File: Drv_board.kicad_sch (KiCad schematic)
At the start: 31 parts, among them J1 USB_B_Micro, J3 OLED_CONN, J4 SWD, J4 WS_LED_0_CONN, J5 WS_LED_1_CONN, J6 SRF-05_CONN, J7 QTR_CONN, SW1 SW_BOOT, U2 STM32F107RCTx, U3 USBLC6-2SC6, Y3 16 MHz

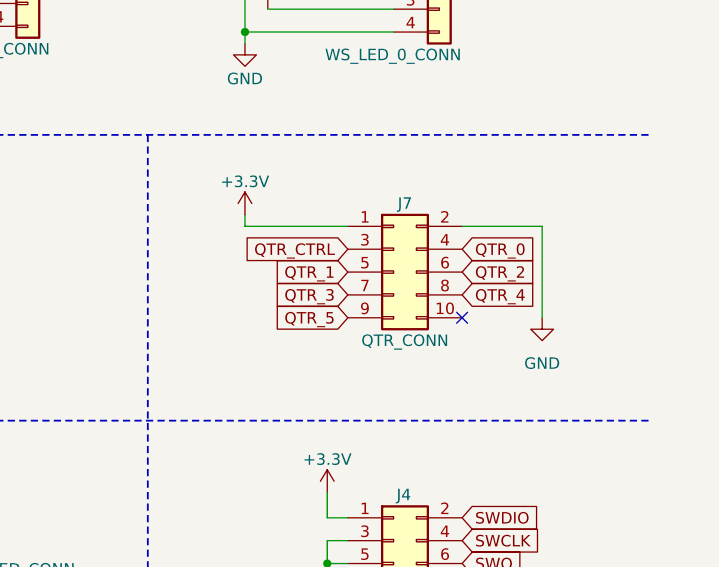
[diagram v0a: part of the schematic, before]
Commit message: more layout
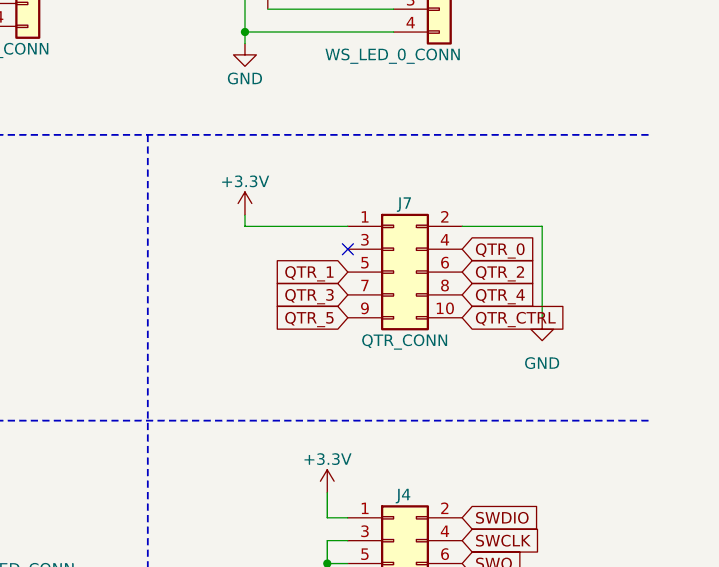
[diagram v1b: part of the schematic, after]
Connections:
- net QTR_CTRL: now also J7.10 (Pin_10); no longer J7.3 (Pin_3)
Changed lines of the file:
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@@
   (no_connect (at 115.57 85.725))
   (no_connect (at 115.57 88.265))
-  (no_connect (at 264.16 102.235))
+  (no_connect (at 251.46 94.615))
   (wire (pts (xy 249.174 124.46) (xy 251.46 124.46))
     (stroke (width 0) (type default))
@@
     )
   )
-  (global_label "QTR_CTRL" (shape input) (at 251.46 94.615 180) (fields_autoplaced)
-    (effects (font (size 1.27 1.27)) (justify right))
-    (property "Intersheetrefs" "${INTERSHEET_REFS}" (at 239.4828 94.615 0)
-      (effects (font (size 1.27 1.27)) (justify right) hide)
+  (global_label "QTR_CTRL" (shape input) (at 264.16 102.235 0) (fields_autoplaced)
+    (effects (font (size 1.27 1.27)) (justify left))
+    (property "Intersheetrefs" "${INTERSHEET_REFS}" (at 276.1372 102.235 0)
+      (effects (font (size 1.27 1.27)) (justify left) hide)
     )
   )

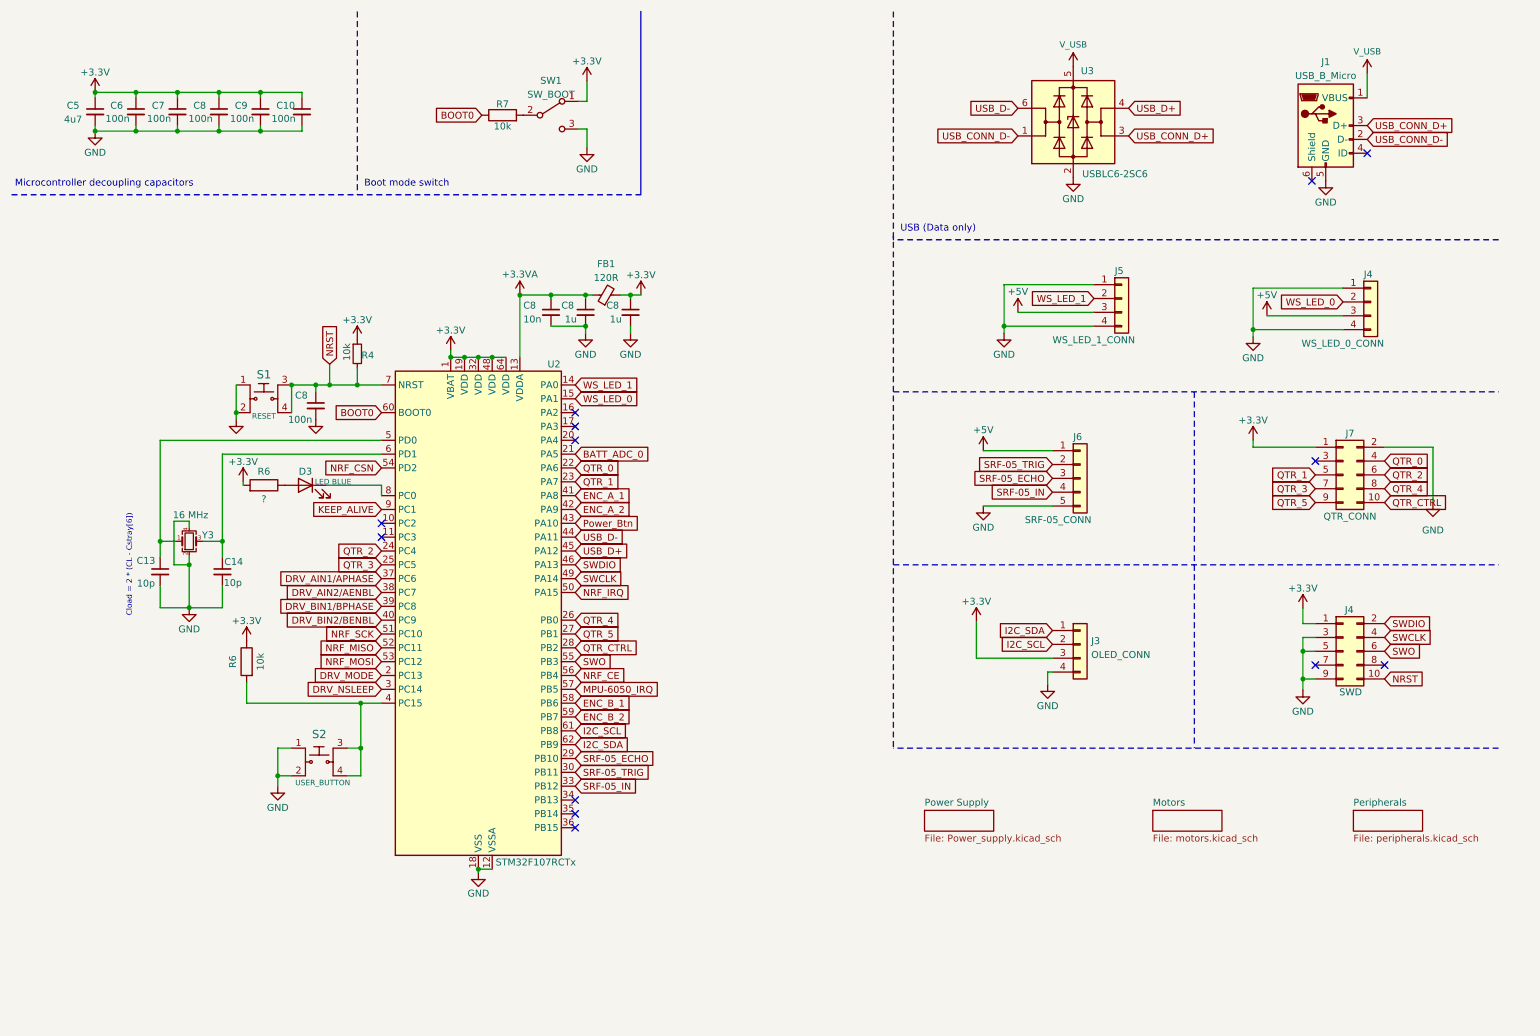
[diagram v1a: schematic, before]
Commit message: layout...
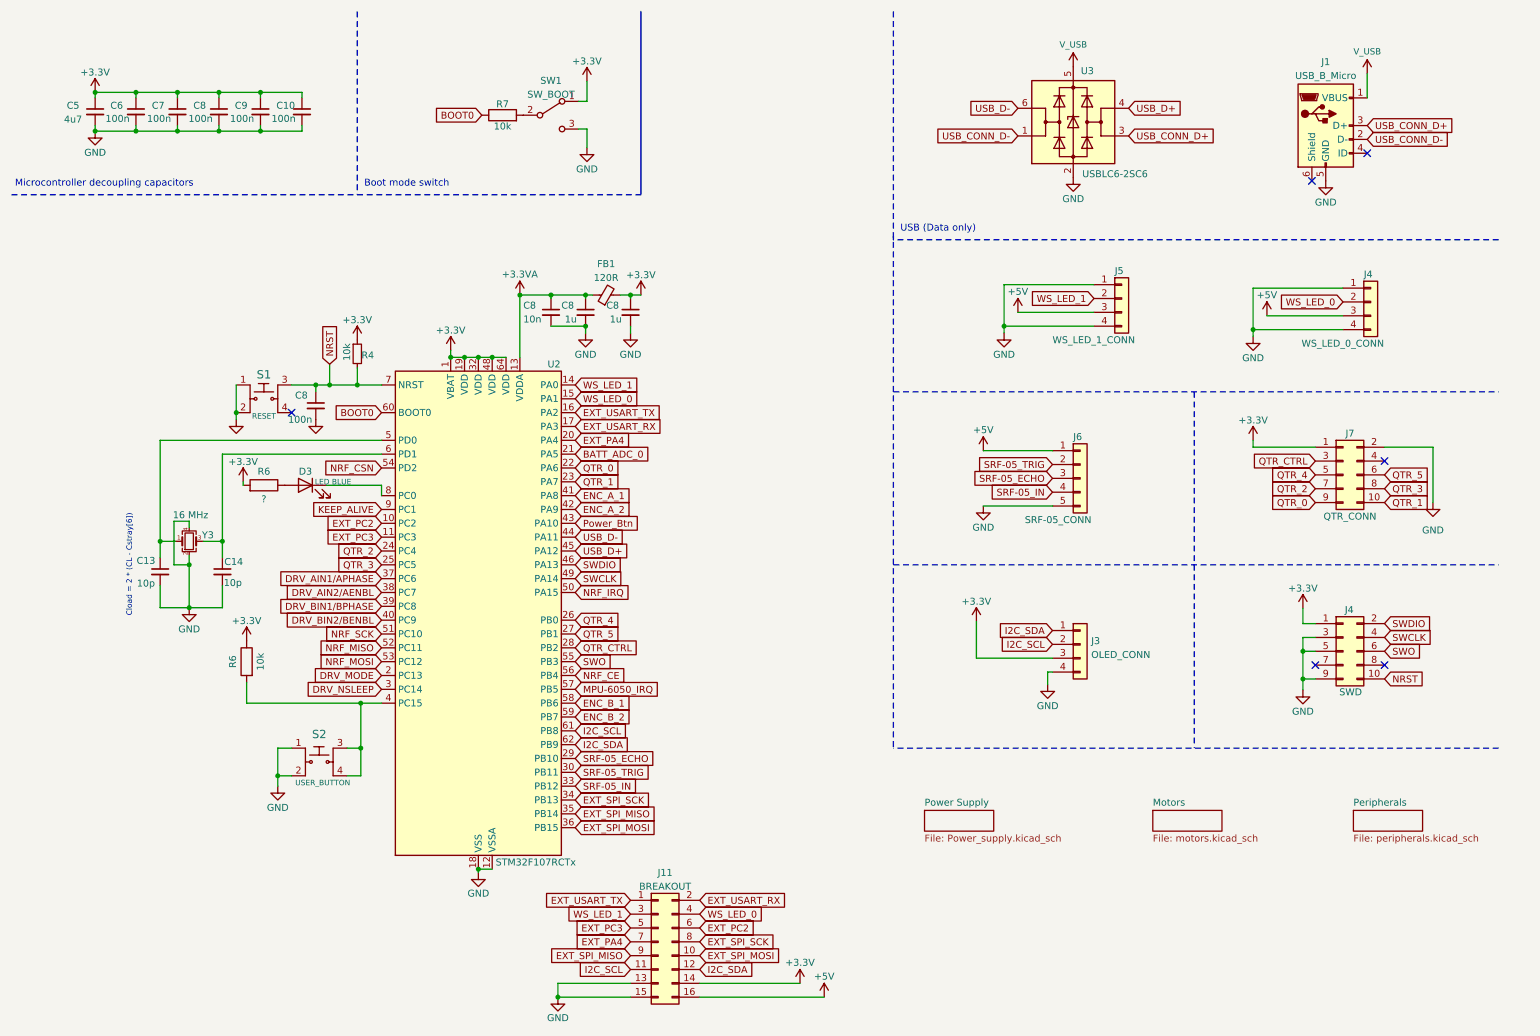
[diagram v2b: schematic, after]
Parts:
- added J11: BREAKOUT, Connector_PinHeader_2.54mm:PinHeader_2x07_P2.54mm_Vertical, symbol Connector_Generic:Conn_02x08_Odd_Even
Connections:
- net +3.3V: now also J11.14 (Pin_14)
- net +5V: now also J11.16 (Pin_16)
- net GND: now also J11.13 (Pin_13), J11.15 (Pin_15)
- net I2C_SCL: now also J11.11 (Pin_11)
- net I2C_SDA: now also J11.12 (Pin_12)
- net NRST: no longer S1.4
- net QTR_0: now also J7.9 (Pin_9); no longer J7.4 (Pin_4)
- net QTR_1: now also J7.10 (Pin_10); no longer J7.5 (Pin_5)
- net QTR_2: now also J7.7 (Pin_7); no longer J7.6 (Pin_6)
- net QTR_3: now also J7.8 (Pin_8); no longer J7.7 (Pin_7)
- net QTR_4: now also J7.5 (Pin_5); no longer J7.8 (Pin_8)
- net QTR_5: now also J7.6 (Pin_6); no longer J7.9 (Pin_9)
- net QTR_CTRL: now also J7.3 (Pin_3); no longer J7.10 (Pin_10)
- net WS_LED_0: now also J11.4 (Pin_4)
- net WS_LED_1: now also J11.3 (Pin_3)
- net EXT_PC2: now reaches U2.10 (PC2)
- net EXT_PC2: now also J11.6 (Pin_6)
- net EXT_PC3: now reaches U2.11 (PC3)
- net EXT_PC3: now also J11.5 (Pin_5)
- net EXT_USART_TX: now reaches U2.16 (PA2)
- net EXT_USART_TX: now also J11.1 (Pin_1)
- net EXT_USART_RX: now reaches U2.17 (PA3)
- net EXT_USART_RX: now also J11.2 (Pin_2)
- net EXT_PA4: now reaches U2.20 (PA4)
- net EXT_PA4: now also J11.7 (Pin_7)
- net EXT_SPI_SCK: now reaches U2.34 (PB13)
- net EXT_SPI_SCK: now also J11.8 (Pin_8)
- net EXT_SPI_MISO: now reaches U2.35 (PB14)
- net EXT_SPI_MISO: now also J11.9 (Pin_9)
- net EXT_SPI_MOSI: now reaches U2.36 (PB15)
- net EXT_SPI_MOSI: now also J11.10 (Pin_10)
- no-connect marks 13 -> 6

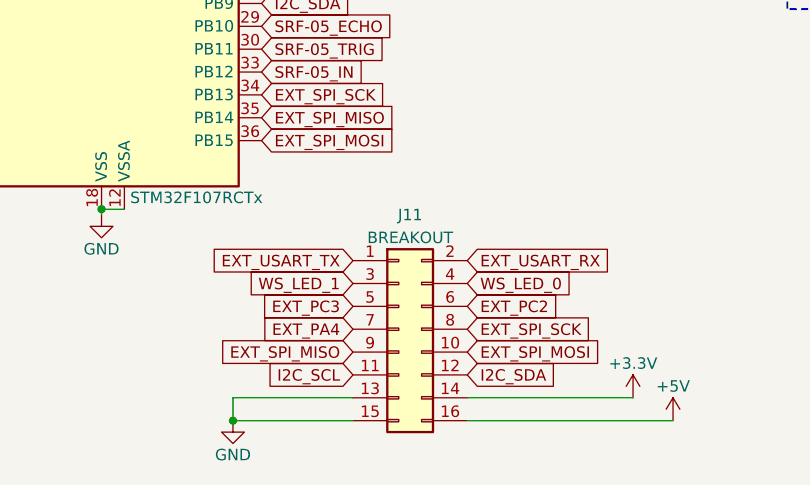
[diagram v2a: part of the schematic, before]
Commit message: layout finalising
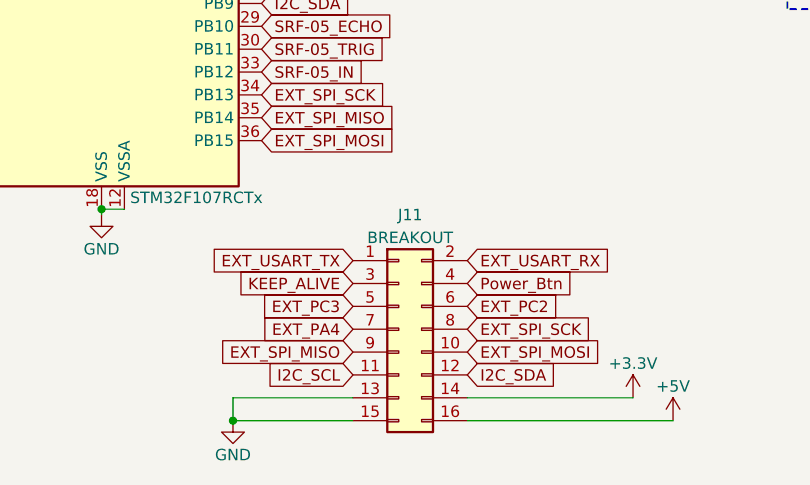
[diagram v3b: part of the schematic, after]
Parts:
- J11: footprint Connector_PinHeader_2.54mm:PinHeader_2x07_P2.54mm_Vertical -> Connector_PinHeader_2.54mm:PinHeader_2x08_P2.54mm_Vertical
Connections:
- net KEEP_ALIVE: now also J11.3 (Pin_3)
- net Power_Btn: now also J11.4 (Pin_4)
- net WS_LED_0: no longer J11.4 (Pin_4)
- net WS_LED_1: no longer J11.3 (Pin_3)
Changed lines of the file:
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@@
+    )
+  )
+  (global_label "Power_Btn" (shape input) (at 138.43 177.8 0) (fields_autoplaced)
+    (effects (font (size 1.27 1.27)) (justify left))
+    (property "Intersheetrefs" "${INTERSHEET_REFS}" (at 151.0724 177.8 0)
+      (effects (font (size 1.27 1.27)) (justify left) hide)
     )
   )
@@
     )
   )
-  (global_label "WS_LED_0" (shape input) (at 138.43 177.8 0) (fields_autoplaced)
-    (effects (font (size 1.27 1.27)) (justify left))
-    (property "Intersheetrefs" "${INTERSHEET_REFS}" (at 150.5885 177.8 0)
-      (effects (font (size 1.27 1.27)) (justify left) hide)
-    )
-  )
   (global_label "QTR_3" (shape input) (at 80.01 113.665 180) (fields_autoplaced)
     (effects (font (size 1.27 1.27)) (justify right))
@@
     )
   )
-  (global_label "WS_LED_1" (shape input) (at 125.73 177.8 180) (fields_autoplaced)
-    (effects (font (size 1.27 1.27)) (justify right))
-    (property "Intersheetrefs" "${INTERSHEET_REFS}" (at 113.5715 177.8 0)
+  (global_label "KEEP_ALIVE" (shape input) (at 125.73 177.8 180) (fields_autoplaced)
+    (effects (font (size 1.27 1.27)) (justify right))
+    (property "Intersheetrefs" "${INTERSHEET_REFS}" (at 112.0595 177.8 0)
       (effects (font (size 1.27 1.27)) (justify right) hide)
     )
@@
       (effects (font (size 1.27 1.27)))
     )
-    (property "Footprint" "Connector_PinHeader_2.54mm:PinHeader_2x07_P2.54mm_Vertical" (at 130.81 182.88 0)
-      (effects (font (size 1.27 1.27)) hide)
-    )
+    (property "Footprint" "Connector_PinHeader_2.54mm:PinHeader_2x08_P2.54mm_Vertical" (at 130.81 182.88 0)
+      (effects (font (size 1.27 1.27)) hide)
+    )

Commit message: Completed PCB v1.0
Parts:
- S1, S2: footprint digikey-footprints:Switch_Tactile_SMD_6x6mm_PTS645 -> digikey-footprints:Switch_Tactile_SMD_6x6mm
- SW1: footprint Jumper:SolderJumper-3_P1.3mm_Open_Pad1.0x1.5mm -> Jumper:SolderJumper-3_P1.3mm_Open_RoundedPad1.0x1.5mm
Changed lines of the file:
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@@
       (effects (font (size 1.27 1.27)))
     )
-    (property "Footprint" "Jumper:SolderJumper-3_P1.3mm_Open_Pad1.0x1.5mm" (at 111.125 31.115 0)
+    (property "Footprint" "Jumper:SolderJumper-3_P1.3mm_Open_RoundedPad1.0x1.5mm" (at 111.125 31.115 0)
       (effects (font (size 1.27 1.27)) hide)
     )
@@
       (effects (font (size 1 1)))
     )
-    (property "Footprint" "digikey-footprints:Switch_Tactile_SMD_6x6mm_PTS645" (at 63.5 78.105 0)
+    (property "Footprint" "digikey-footprints:Switch_Tactile_SMD_6x6mm" (at 63.5 78.105 0)
       (effects (font (size 1.524 1.524)) (justify left) hide)
     )
@@
       (effects (font (size 1 1)))
     )
-    (property "Footprint" "digikey-footprints:Switch_Tactile_SMD_6x6mm_PTS645" (at 73.66 144.78 0)
-      (effects (font (size 1.524 1.524)) (justify left) hide)
-    )
+    (property "Footprint" "digikey-footprints:Switch_Tactile_SMD_6x6mm" (at 73.66 144.78 0)
+      (effects (font (size 1.524 1.524)) (justify left) hide)
+    )
